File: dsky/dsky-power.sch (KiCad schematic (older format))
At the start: 18 parts, among them Q9 PMOS, U27 TPS61020

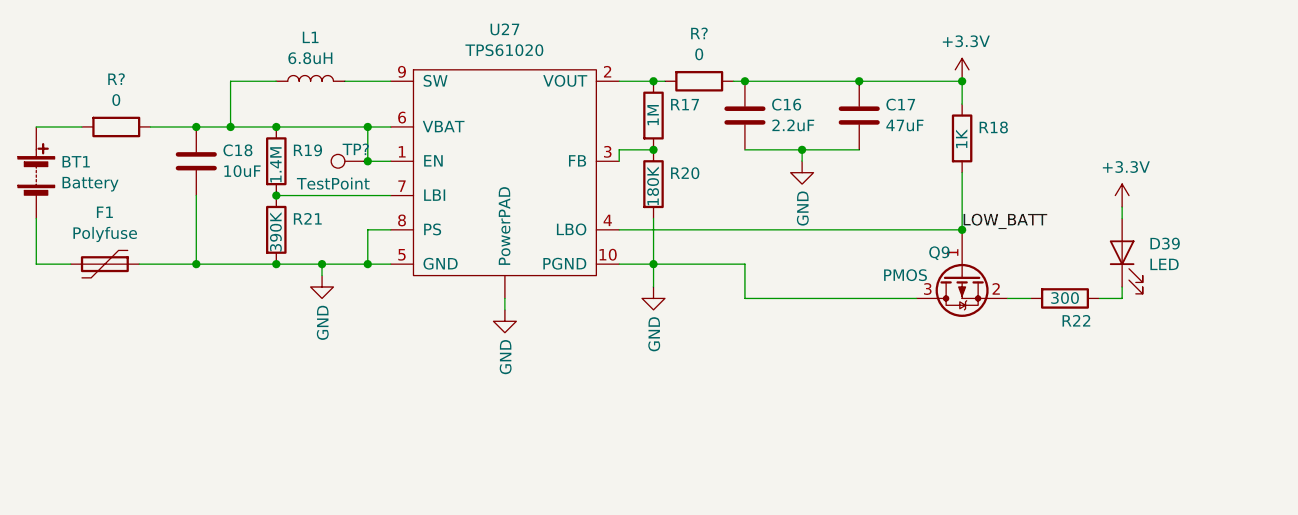
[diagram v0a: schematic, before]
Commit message: this hard drive is dying
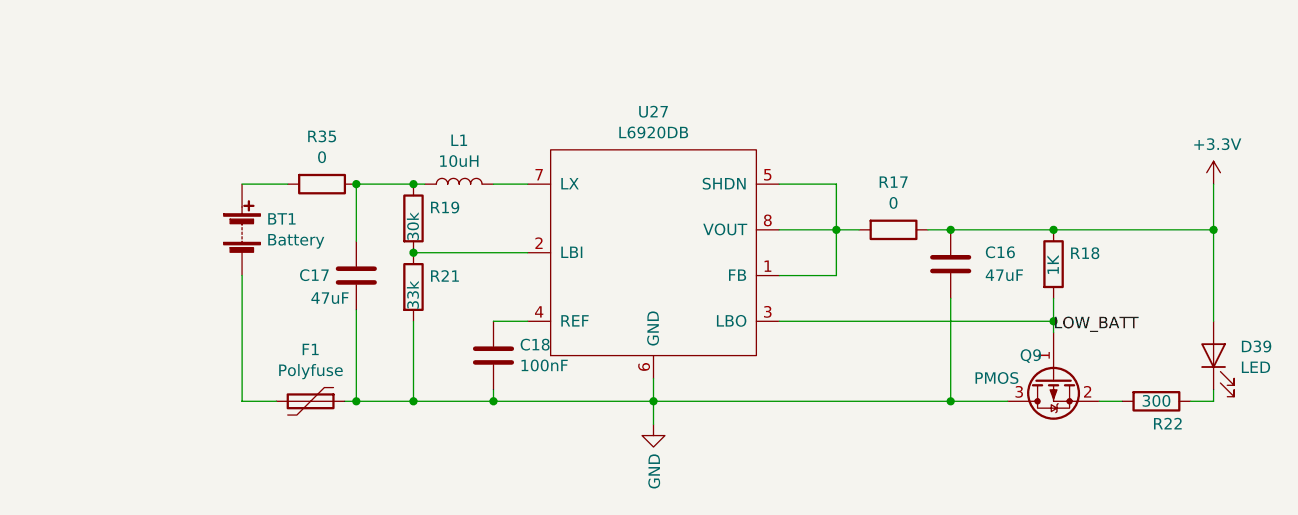
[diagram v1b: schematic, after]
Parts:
- removed R20: 180K, Resistor_SMD:R_0603_1608Metric, symbol Device:R
- removed R?: 0, symbol Device:R
- removed TP?: TestPoint, symbol Connector:TestPoint
- removed U27: TPS61020, symbol dsky:TPS61020
- added U27: L6920DB, Package_SO:MSOP-8_3x3mm_P0.65mm, symbol dsky:L6920DB
- C16: value 2.2uF -> 47uF; footprint Capacitor_SMD:C_0805_2012Metric -> Capacitor_SMD:C_1206_3216Metric
- C18: value 10uF -> 100nF; footprint Capacitor_SMD:C_1206_3216Metric -> Capacitor_SMD:C_0402_1005Metric
- L1: value 6.8uH -> 10uH
- R17: value 1M -> 0; footprint Resistor_SMD:R_0603_1608Metric -> Resistor_SMD:R_0402_1005Metric
- R18: footprint Resistor_SMD:R_0603_1608Metric -> Resistor_SMD:R_0402_1005Metric
- R19: value 1.4M -> 30k; footprint Resistor_SMD:R_0603_1608Metric -> Resistor_SMD:R_0402_1005Metric
- R21: value 390K -> 33k; footprint Resistor_SMD:R_0603_1608Metric -> Resistor_SMD:R_0402_1005Metric
- R22: footprint Resistor_SMD:R_0805_2012Metric -> Resistor_SMD:R_0603_1608Metric
- R35: renamed from R?; footprint (none) -> Resistor_SMD:R_0402_1005Metric
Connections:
- net +3V3: now also R17.1; no longer C17.1
- net GND: now also U27.6 (GND)
- net LOW_BATT: now also U27.3 (LBO)
- net at L1.1, R19.1, R35.1: now also C17.1; no longer C18.1
- net at R17.2: now also U27.1 (FB), U27.5 (SHDN), U27.8 (VOUT)
- net at R19.2, R21.1: now also U27.2 (LBI)
- net at L1.2: now also U27.7 (LX)
- new net: C18.1, U27.4 (REF)
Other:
- moved on the sheet: BT1, C17, D39, F1, L1, Q9, R19, R21, R22, R35
